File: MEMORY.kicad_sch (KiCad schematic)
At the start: 5 parts, among them U2 ICE40HX8K-BG121, U7 S27KL0641

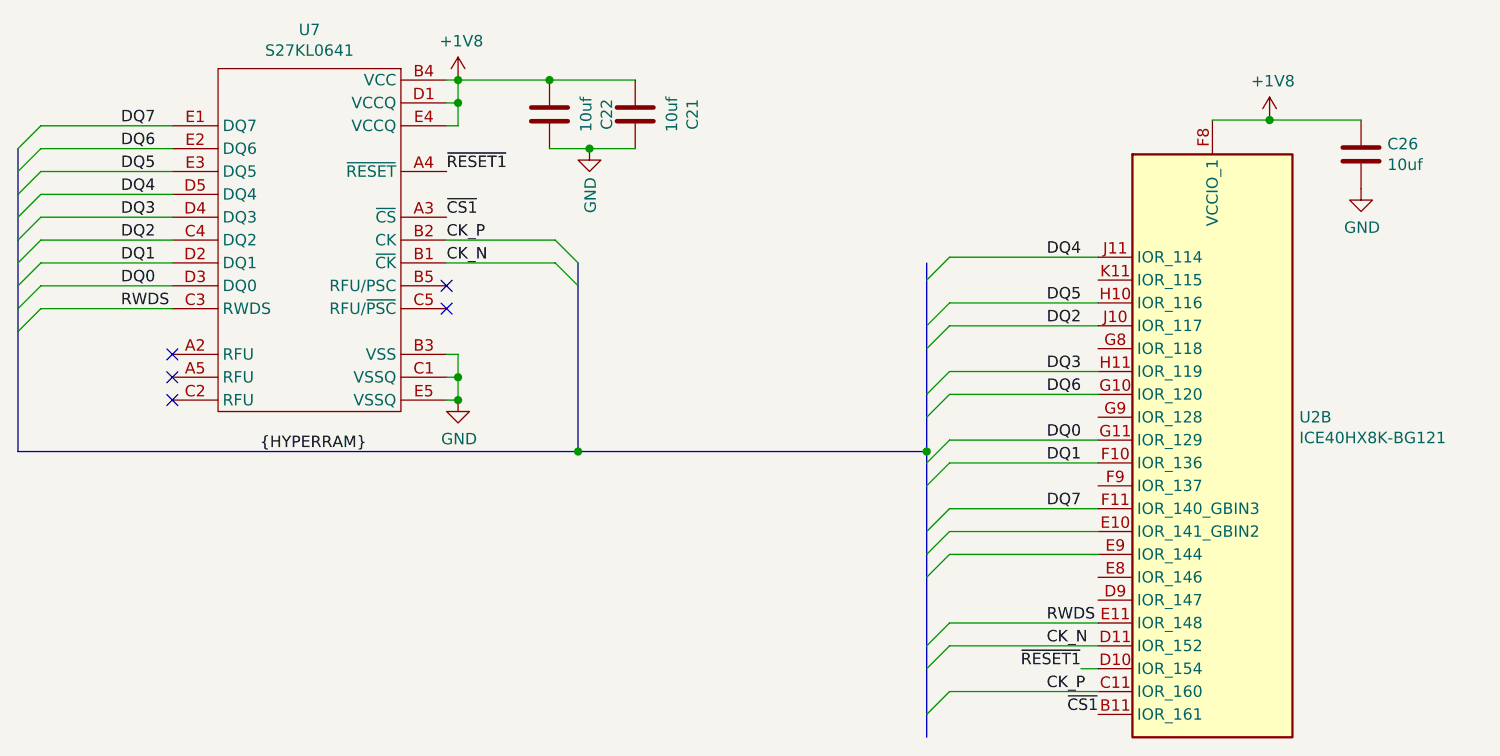
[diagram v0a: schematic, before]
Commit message: Routing changes, pullups, etc
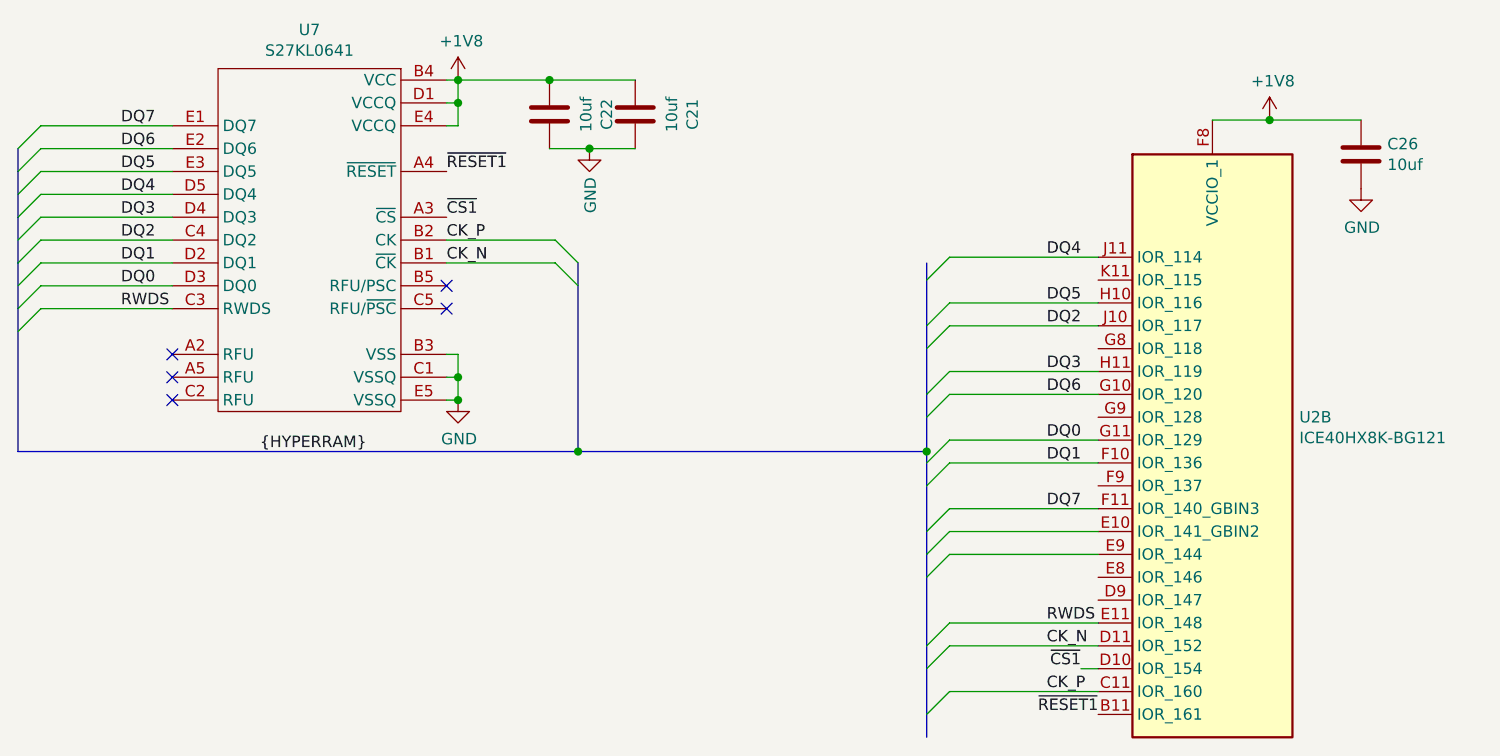
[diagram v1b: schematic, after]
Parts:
- C21, C22, C26, U2: Source (none) -> ANY
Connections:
- net ~CS1: now also U2.D10 (IOR_154); no longer U2.B11 (IOR_161)
- net ~RESET1: now also U2.B11 (IOR_161); no longer U2.D10 (IOR_154)
